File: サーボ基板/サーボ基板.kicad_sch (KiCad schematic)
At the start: 21 parts, among them J1 Conn_01x02, J2 Conn_01x03, J3 Conn_01x03, J4 Conn_01x03, J5 Conn_01x03, U1 SeeeduinoXIAO RP2040

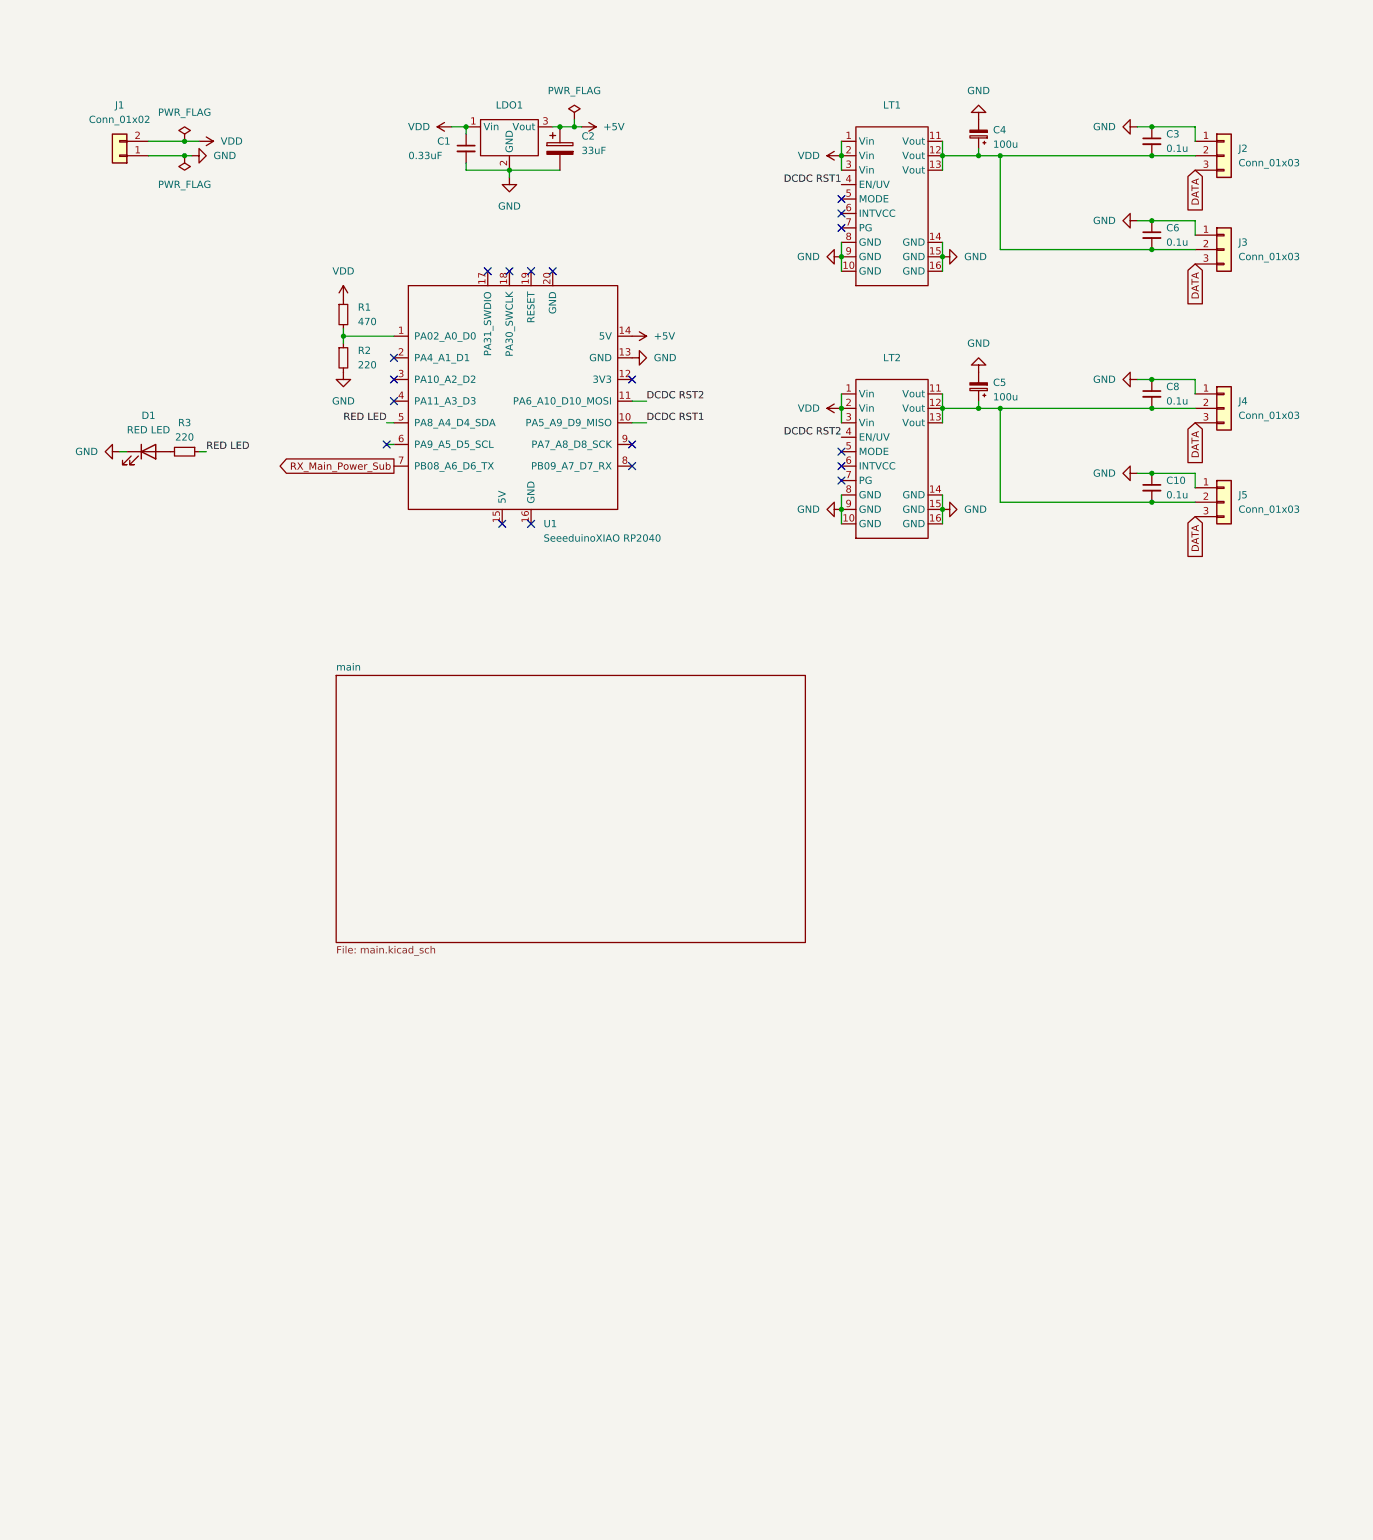
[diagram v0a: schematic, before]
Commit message: main
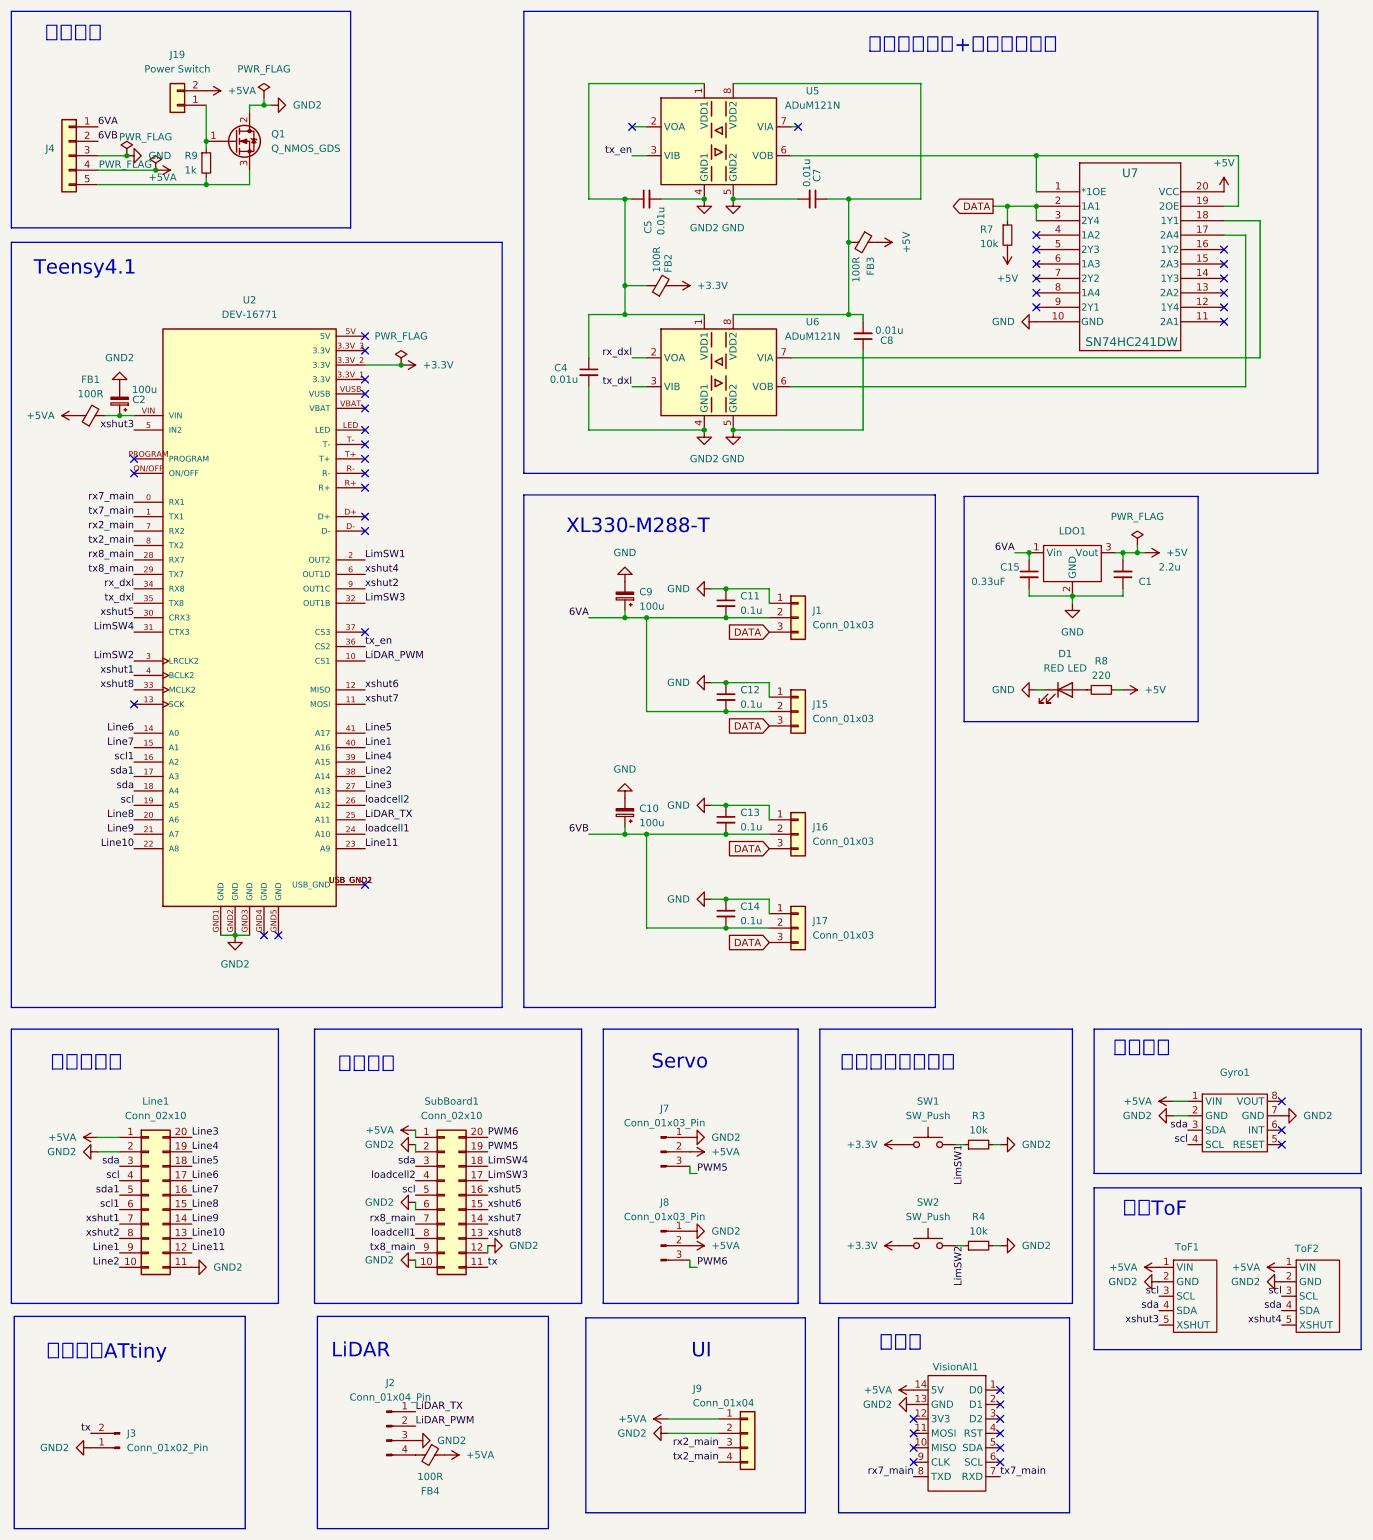
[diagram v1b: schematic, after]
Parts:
- removed C10, C3, C6: 0.1u, Capacitor_SMD:C_0603_1608Metric_Pad1.08x0.95mm_HandSolder, symbol Device:C_Small
- removed C2: 33uF, Capacitor_THT:CP_Radial_D5.0mm_P2.00mm, symbol Device:C_Polarized
- removed C4, C5: 100u, Capacitor_THT:CP_Radial_D6.3mm_P2.50mm, symbol Device:C_Polarized_Small
- removed J1: Conn_01x02, Connector_AMASS:AMASS_XT30PW-M_1x02_P2.50mm_Horizontal, symbol Connector_Generic:Conn_01x02
- removed J2, J3: Conn_01x03, Connector_JST:JST_EH_S3B-EH_1x03_P2.50mm_Horizontal, symbol Connector_Generic:Conn_01x03
- removed J4, J5: Conn_01x03, Connector_JST:JST_EH_B3B-EH-A_1x03_P2.50mm_Vertical, symbol Connector_Generic:Conn_01x03
- removed LT1, LT2: ~, LT8640:LT8640, symbol LT8640:LT8640
- removed R1: 470, Resistor_SMD:R_0603_1608Metric_Pad0.98x0.95mm_HandSolder, symbol Device:R_Small
- removed R2: 220, Resistor_SMD:R_0603_1608Metric_Pad0.98x0.95mm_HandSolder, symbol Device:R_Small
- removed U1: SeeeduinoXIAO RP2040, XIAO RP2040:XIAO RP2040, symbol Seeeduino XIAO:SeeeduinoXIAO
- added C10, C2, C9: 100u, Capacitor_THT:CP_Radial_D6.3mm_P2.50mm, symbol Device:C_Polarized_Small
- added C11, C12, C13, C14: 0.1u, Capacitor_SMD:C_0603_1608Metric_Pad1.08x0.95mm_HandSolder, symbol Device:C_Small
- added C15: 0.33uF, Capacitor_SMD:C_0603_1608Metric_Pad1.08x0.95mm_HandSolder, symbol Device:C_Small
- added C4, C5, C7: 0.01u, Capacitor_SMD:C_0603_1608Metric_Pad1.08x0.95mm_HandSolder, symbol Device:C_Small
- added FB1, FB2, FB3, FB4: 100R, Inductor_SMD:L_Walsin_WLFM201209x, symbol Device:FerriteBead_Small
- added Gyro1: ~, MyLibrary:BNO055, symbol MyLibrary:BNO055
- added J1, J15, J16, J17: Conn_01x03, Connector_JST:JST_EH_S3B-EH_1x03_P2.50mm_Horizontal, symbol Connector_Generic:Conn_01x03
- added J19: Power Switch, Connector_JST:JST_XH_B2B-XH-A_1x02_P2.50mm_Vertical, symbol Connector_Generic:Conn_01x02
- added J2: Conn_01x04_Pin, Connector_PinHeader_2.54mm:PinHeader_1x04_P2.54mm_Vertical, symbol Connector:Conn_01x04_Pin
- added J3: Conn_01x02_Pin, Connector_JST:JST_XH_S2B-XH-A_1x02_P2.50mm_Horizontal, symbol Connector:Conn_01x02_Pin
- added J4: PWR OUT, Connector_JST:JST_VH_B5PS-VH_1x05_P3.96mm_Horizontal, symbol Connector_Generic:Conn_01x05
- added J7, J8: Conn_01x03_Pin, Connector_PinHeader_2.54mm:PinHeader_1x03_P2.54mm_Vertical, symbol Connector:Conn_01x03_Pin
- added J9: Conn_01x04, Connector_JST:JST_XH_B4B-XH-A_1x04_P2.50mm_Vertical, symbol Connector_Generic:Conn_01x04
- added Line1, SubBoard1: Conn_02x10, Connector_PinHeader_2.54mm:PinHeader_2x10_P2.54mm_Vertical, symbol Connector_Generic:Conn_02x10_Counter_Clockwise
- added Q1: Q_NMOS_GDS, Package_TO_SOT_SMD:TO-252-2, symbol Device:Q_NMOS_GDS
- added R4, R7: 10k, Resistor_SMD:R_0603_1608Metric_Pad0.98x0.95mm_HandSolder, symbol Device:R_Small
- added R8: 220, Resistor_SMD:R_0603_1608Metric_Pad0.98x0.95mm_HandSolder, symbol Device:R_Small
- added R9: 1k, Resistor_SMD:R_0603_1608Metric_Pad0.98x0.95mm_HandSolder, symbol Device:R_Small
- added SW1, SW2: SW_Push, Connector_JST:JST_XH_B2B-XH-A_1x02_P2.50mm_Vertical, symbol Switch:SW_Push
- added ToF1, ToF2: ~, ToF:GY530, symbol ToF:GY530
- added U2: DEV-16771, DEV-16771:MODULE_DEV-16771, symbol DEV-16771:DEV-16771
- added U5, U6: ADuM121N, MyLibrary:SOP-8_DIP, symbol Isolator:ADuM121N
- added U7: SN74HC241DW, Package_DIP:CERDIP-20_W7.62mm_SideBrazed_Socket, symbol 2024-09-28_15-43-53:SN74HC241DW
- added VisionAI1: ~, MyLibrary:Grove Vision AI V2, symbol MyLibrary:Grove_Vision_AI_V2
- C1: value 0.33uF -> 2.2u; footprint Capacitor_THT:C_Disc_D3.0mm_W1.6mm_P2.50mm -> Capacitor_SMD:C_0603_1608Metric_Pad1.08x0.95mm_HandSolder
- C8: value 0.1u -> 0.01u
- LDO1: footprint Package_TO_SOT_THT:TO-220-3_Horizontal_TabDown -> Package_TO_SOT_SMD:TO-252-2
- R3: value 220 -> 10k
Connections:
- net +5V: now also C1.2, FB3.1, R7.2, R8.1, U7.20 (VCC)
- net DATA: now also J1.3 (Pin_3), J15.3 (Pin_3), J16.3 (Pin_3), J17.3 (Pin_3), R7.1, U7.2 (1A1), U7.3 (2Y4)
- net GND: now also C1.1, C10.2, C11.1, C12.1, C13.1, C14.1, C15.2, C7.2, C9.2, J1.1 (Pin_1), J15.1 (Pin_1), J16.1 (Pin_1), J17.1 (Pin_1), J4.3 (Pin_3), U5.5 (GND2), U6.5 (GND2), U7.10 (GND); no longer C1.2
- net at C8.2: now also C7.1, FB3.2, U5.8 (VDD2), U6.8 (VDD2)
- net at D1.2 (A): now also R8.2; no longer R3.2
- net RED LED renamed LimSW1
- net LimSW1: now also SW1.2, U2.2 (OUT2)
- net VDD renamed 6VA
- net 6VA: now also C11.2, C12.2, C15.1, C9.1, J1.2 (Pin_2), J15.2 (Pin_2), J4.1 (Pin_1); no longer C1.1
- new net: C4.1, C5.1, FB2.1, U5.1 (VDD1), U6.1 (VDD1)
- new net: J19.1 (Pin_1), Q1.1 (G), R9.1
- new net: J4.5 (Pin_5), Q1.3 (S), R9.2
- new net: U2.USB_GND1 (USB_GND), U2.USB_GND2 (USB_GND)
- new net: C2.1, FB1.2, U2.VIN
- new net: U6.6 (VOB), U7.17 (2A4)
- new net: U6.7 (VIA), U7.18 (1Y1)
- new net: FB4.2, J2.4 (Pin_4)
- new net: U5.6 (VOB), U7.1 (*1OE), U7.19 (2OE)
- new net +3.3V: FB2.2, SW1.1, SW2.1, U2.3.3V_2 (3.3V)
- new net +5VA: FB1.1, FB4.1, Gyro1.1 (VIN), J19.2 (Pin_2), J4.4 (Pin_4), J7.2 (Pin_2), J8.2 (Pin_2), J9.1 (Pin_1), Line1.1 (Pin_1), SubBoard1.1 (Pin_1), ToF1.1 (VIN), ToF2.1 (VIN), VisionAI1.14 (5V)
- new net 6VB: C10.1, C13.2, C14.2, J16.2 (Pin_2), J17.2 (Pin_2), J4.2 (Pin_2)
- new net GND2: C2.2, C4.2, C5.2, Gyro1.2 (GND), Gyro1.7 (GND), J2.3 (Pin_3), J3.1 (Pin_1), J7.1 (Pin_1), J8.1 (Pin_1), J9.2 (Pin_2), Line1.11 (Pin_11), Line1.2 (Pin_2), Q1.2 (D), R3.2, R4.2, SubBoard1.10 (Pin_10), SubBoard1.12 (Pin_12), SubBoard1.2 (Pin_2), SubBoard1.6 (Pin_6), ToF1.2 (GND), ToF2.2 (GND), U2.GND1 (GND), U2.GND2 (GND), U2.GND3 (GND), U5.4 (GND1), U6.4 (GND1), VisionAI1.13 (GND)
- new net LiDAR_PWM: J2.2 (Pin_2), U2.10 (CS1)
- new net LiDAR_TX: J2.1 (Pin_1), U2.25 (A11)
- new net LimSW2: R4.1, SW2.2, U2.3 (LRCLK2)
- new net LimSW3: SubBoard1.17 (Pin_17), U2.32 (OUT1B)
- new net LimSW4: SubBoard1.18 (Pin_18), U2.31 (CTX3)
- new net Line1: Line1.9 (Pin_9), U2.40 (A16)
- new net Line10: Line1.13 (Pin_13), U2.22 (A8)
- new net Line11: Line1.12 (Pin_12), U2.23 (A9)
- new net Line2: Line1.10 (Pin_10), U2.38 (A14)
- new net Line3: Line1.20 (Pin_20), U2.27 (A13)
- new net Line4: Line1.19 (Pin_19), U2.39 (A15)
- new net Line5: Line1.18 (Pin_18), U2.41 (A17)
- new net Line6: Line1.17 (Pin_17), U2.14 (A0)
- new net Line7: Line1.16 (Pin_16), U2.15 (A1)
- new net Line8: Line1.15 (Pin_15), U2.20 (A6)
- new net Line9: Line1.14 (Pin_14), U2.21 (A7)
- new net PWM5: J7.3 (Pin_3), SubBoard1.19 (Pin_19)
- new net PWM6: J8.3 (Pin_3), SubBoard1.20 (Pin_20)
- new net loadcell1: SubBoard1.8 (Pin_8), U2.24 (A10)
- new net loadcell2: SubBoard1.4 (Pin_4), U2.26 (A12)
- new net rx2_main: J9.3 (Pin_3), U2.7 (RX2)
- new net rx7_main: U2.0 (RX1), VisionAI1.8 (TXD)
- new net rx8_main: SubBoard1.7 (Pin_7), U2.28 (RX7)
- new net rx_dxl: U2.34 (RX8), U6.2 (VOA)
- new net scl: Gyro1.4 (SCL), Line1.4 (Pin_4), SubBoard1.5 (Pin_5), ToF1.3 (SCL), ToF2.3 (SCL), U2.19 (A5)
- new net scl1: Line1.6 (Pin_6), U2.16 (A2)
- new net sda: Gyro1.3 (SDA), Line1.3 (Pin_3), SubBoard1.3 (Pin_3), ToF1.4 (SDA), ToF2.4 (SDA), U2.18 (A4)
- new net sda1: Line1.5 (Pin_5), U2.17 (A3)
- new net tx: J3.2 (Pin_2), SubBoard1.11 (Pin_11)
- new net tx2_main: J9.4 (Pin_4), U2.8 (TX2)
- new net tx7_main: U2.1 (TX1), VisionAI1.7 (RXD)
- new net tx8_main: SubBoard1.9 (Pin_9), U2.29 (TX7)
- new net tx_dxl: U2.35 (TX8), U6.3 (VIB)
- new net tx_en: U2.36 (CS2), U5.3 (VIB)
- new net xshut1: Line1.7 (Pin_7), U2.4 (BCLK2)
- new net xshut2: Line1.8 (Pin_8), U2.9 (OUT1C)
- new net xshut3: ToF1.5 (XSHUT), U2.5 (IN2)
- new net xshut4: ToF2.5 (XSHUT), U2.6 (OUT1D)
- new net xshut5: SubBoard1.16 (Pin_16), U2.30 (CRX3)
- new net xshut6: SubBoard1.15 (Pin_15), U2.12 (MISO)
- new net xshut7: SubBoard1.14 (Pin_14), U2.11 (MOSI)
- new net xshut8: SubBoard1.13 (Pin_13), U2.33 (MCLK2)
- no-connect marks 19 -> 46
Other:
- removed sheet main
- note added: "LiDAR"
- note added: "Servo"
- note added: "Teensy4.1"
- note added: "UI"
- note added: "XL330-M288-T"
- note added: "カメラ"
- note added: "サブ基板"
- note added: "シリアル変換+アイソレート"
- note added: "ジャイロ"
- note added: "ライン基板"
- note added: "リミットスイッチ"
- note added: "側面ToF"
- note added: "電源入力"
- note added: "電源基板ATtiny"
